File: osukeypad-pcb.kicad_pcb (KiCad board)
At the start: 2 copper layers, 93.7 x 38.1 mm, 24 parts, among them SW1 SW_Push, U1 ATmega32U4-AU, Y1 16MHz

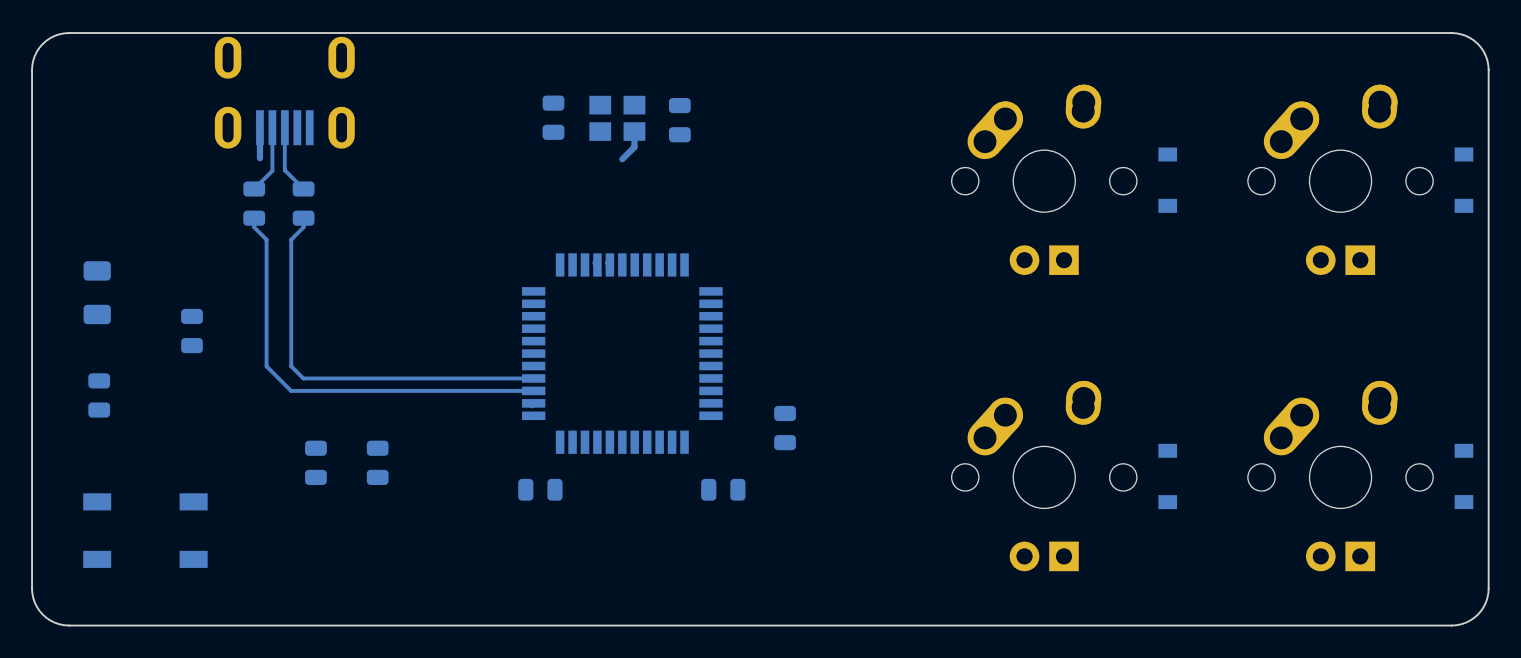
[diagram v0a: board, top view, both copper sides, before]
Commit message: osupad-update-3
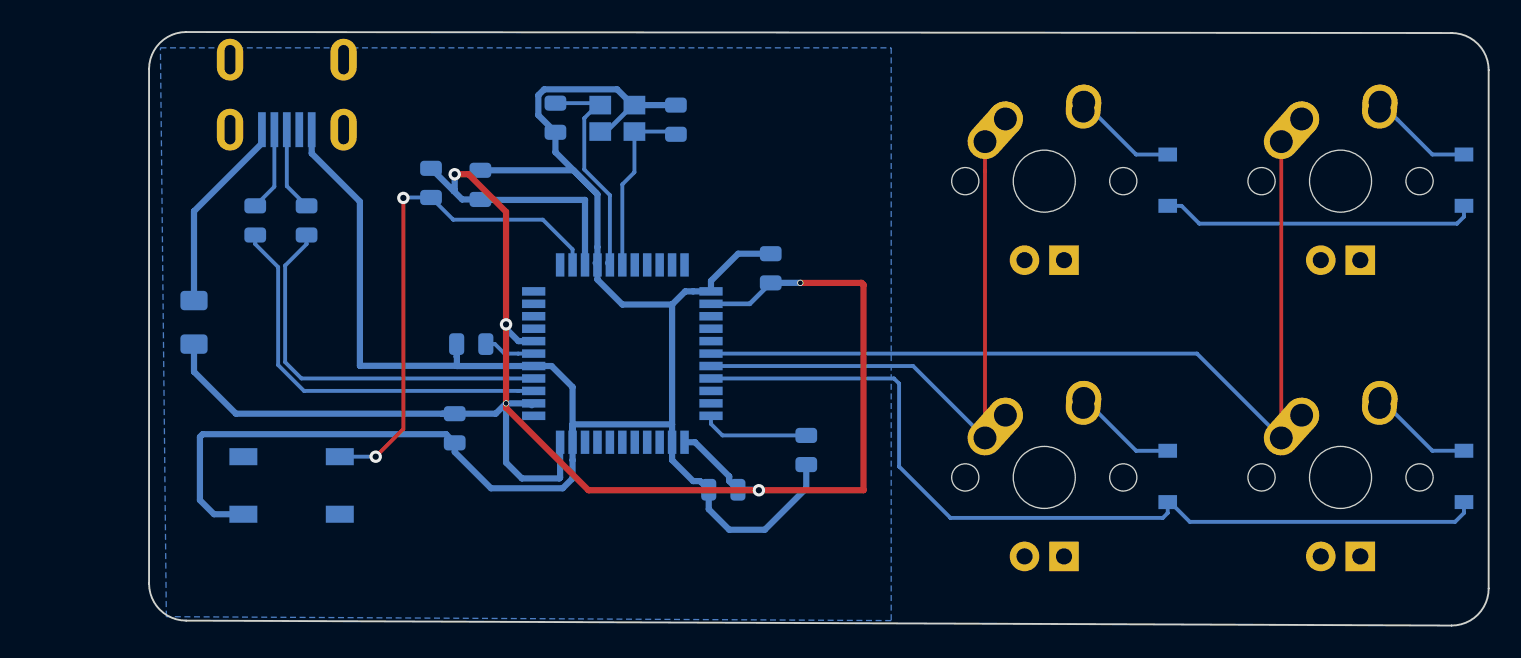
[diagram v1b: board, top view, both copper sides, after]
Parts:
- moved C3 43.9 mm to (76.1, 67.5), turned to 90 degrees
- moved C1 20.8 mm to (57.4, 62.2)
- moved R3 18.1 mm to (54.2, 62.0)
- moved C7 10.4 mm to (56.8, 72.4), turned to 180 degrees
- moved SW1 9.84 mm to (45.3, 81.5)
- moved F1 6.51 mm to (39.0, 71.0)
- moved C2 5.43 mm to (55.8, 77.8), turned to 270 degrees
- moved R4 1.96 mm to (78.4, 79.2)
- moved R2 1.10 mm to (46.2, 64.4)
- moved R1 1.08 mm to (42.9, 64.4)
- moved C4 0.26 mm to (70.0, 58.0)
- moved USB1 0.18 mm to (45.0, 54.1)
- moved C5 0.13 mm to (62.2, 57.8)
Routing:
- net GND: track 2.19 -> 151.4 mm
- net +5V: track 0.36 -> 126.4 mm, vias 0 -> 5
- net COL1: track 0.01 -> 58.0 mm
- net ROW1: track 0.15 -> 57.6 mm
- net COL0: track 0.01 -> 38.6 mm
- net Net-(R3-Pad2): track 0.15 -> 33.0 mm, vias 0 -> 2
- net ROW0: track 0.00 -> 20.4 mm
- net Net-(C5-Pad1): track 0.82 -> 15.2 mm
- net VCC: track 2.84 -> 12.8 mm
- net Net-(C4-Pad1): track 2.39 -> 11.9 mm
- net Net-(R4-Pad2): track 0.00 -> 6.96 mm
- net Net-(D2-Pad2): track 0.82 -> 7.61 mm
- net Net-(D4-Pad2): track 0.82 -> 7.61 mm
- net Net-(D3-Pad2): track 0.82 -> 7.61 mm
- net Net-(D1-Pad2): track 0.82 -> 7.41 mm
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- added copper zone on B.Cu, net GND
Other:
- board size 93.7 x 38.1 mm -> 86.1 x 38.2 mm
- net class Power: trace_width 0.25 -> 0.4
